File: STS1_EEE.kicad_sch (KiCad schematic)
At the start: 20 parts, among them J1 2477, J2 Conn_02x20_Odd_Even, J3 Conn_02x20_Odd_Even, SW1 SW_SPST, U1 coordinate_system, U10 ST_Logo

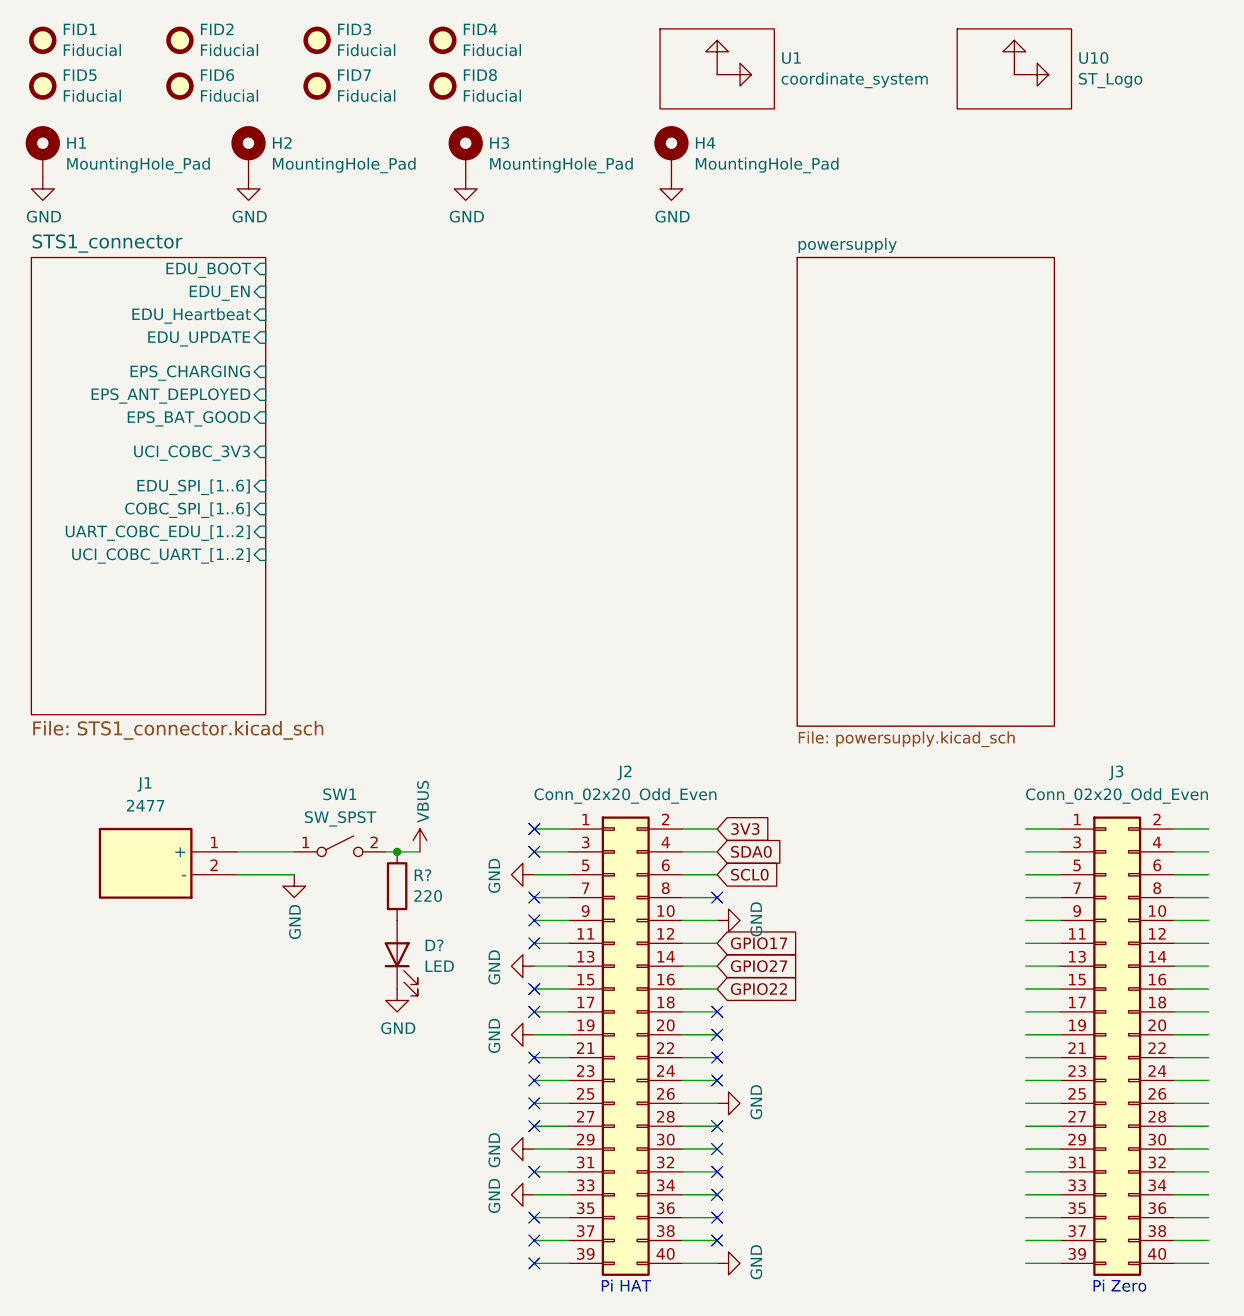
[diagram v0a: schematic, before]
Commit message: Label RasPi Zero W pin header
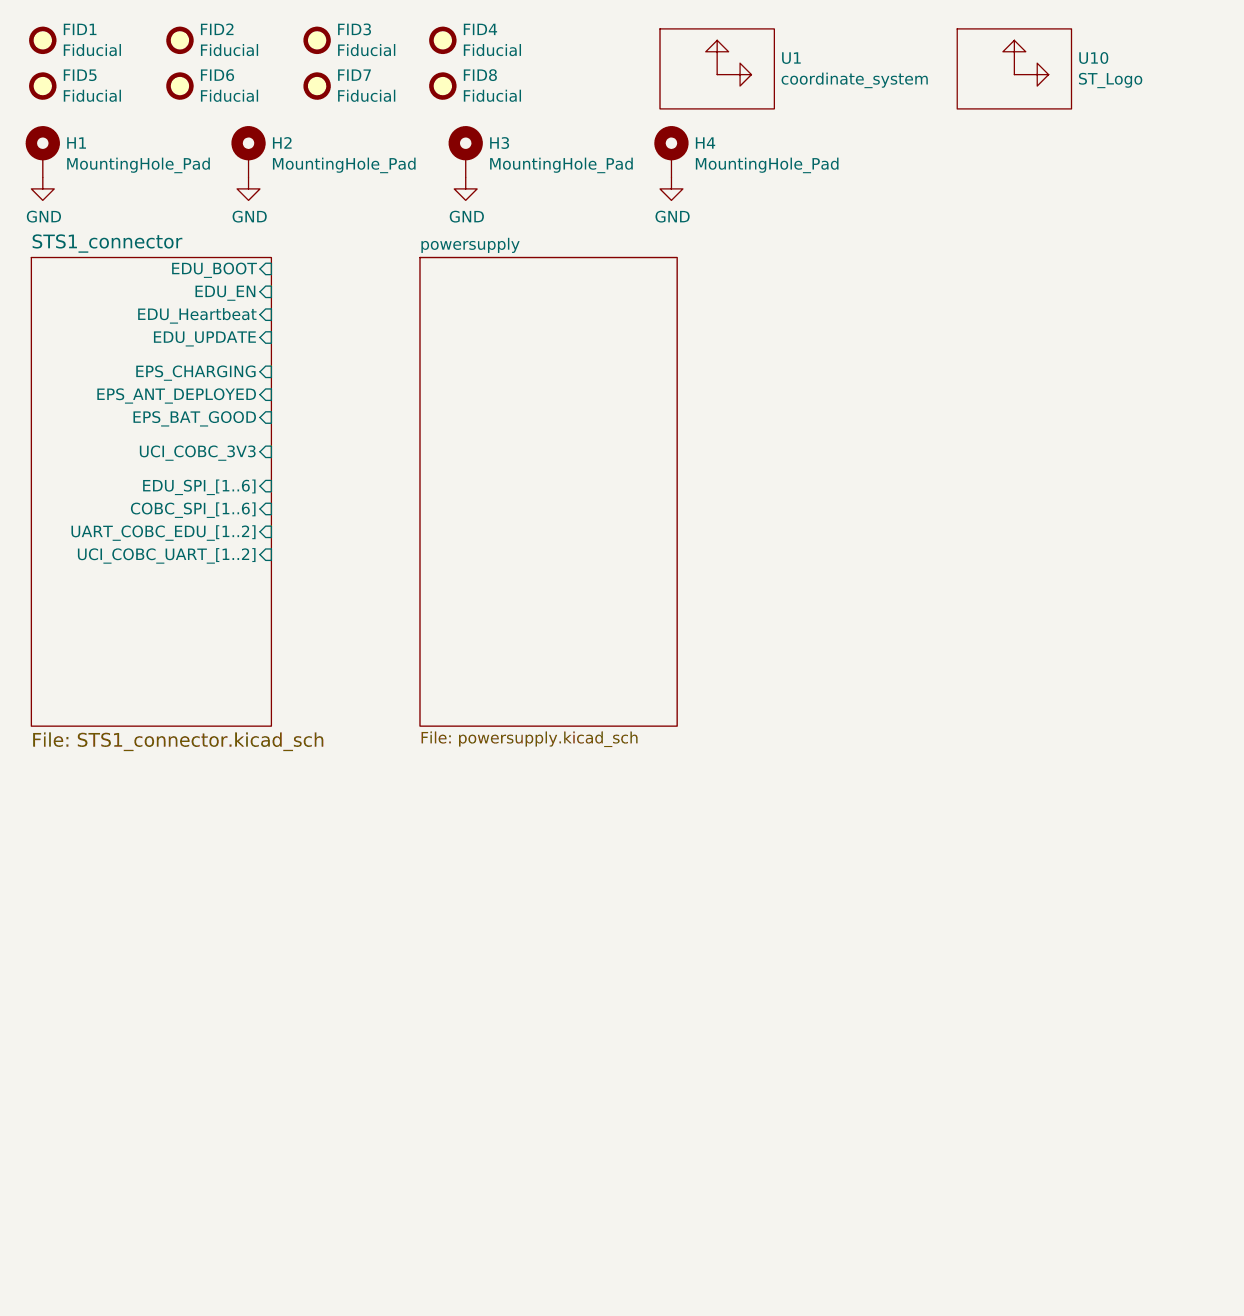
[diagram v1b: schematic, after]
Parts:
- removed D?: LED, LED_SMD:LED_0805_2012Metric, symbol Device:LED
- removed J1: 2477, 2477, symbol STS1_EEE_lib:2477
- removed J2, J3: Conn_02x20_Odd_Even, symbol Connector_Generic:Conn_02x20_Odd_Even
- removed R?: 220, Resistor_SMD:R_0603_1608Metric, symbol Device:R
- removed SW1: SW_SPST, symbol Switch:SW_SPST
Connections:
- no-connect marks 26 -> 0
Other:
- note removed: "Pi HAT"
- note removed: "Pi Zero"
